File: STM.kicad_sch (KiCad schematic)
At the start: 29 parts, among them J7 PIN HEADER 2.54MM PITCH STR D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, U1 STM32L433CCU6, X1 CRYSTAL 32.0000MHZ 10PF SMD

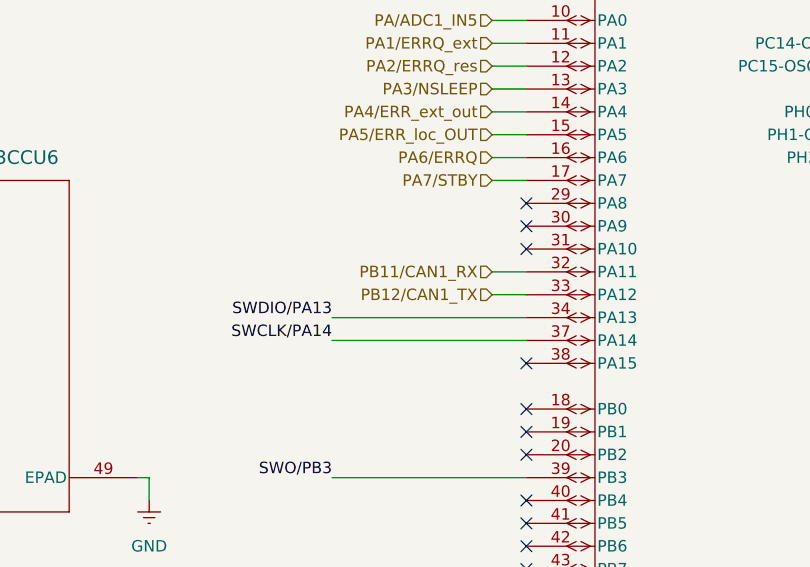
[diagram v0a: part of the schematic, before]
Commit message: minor changes
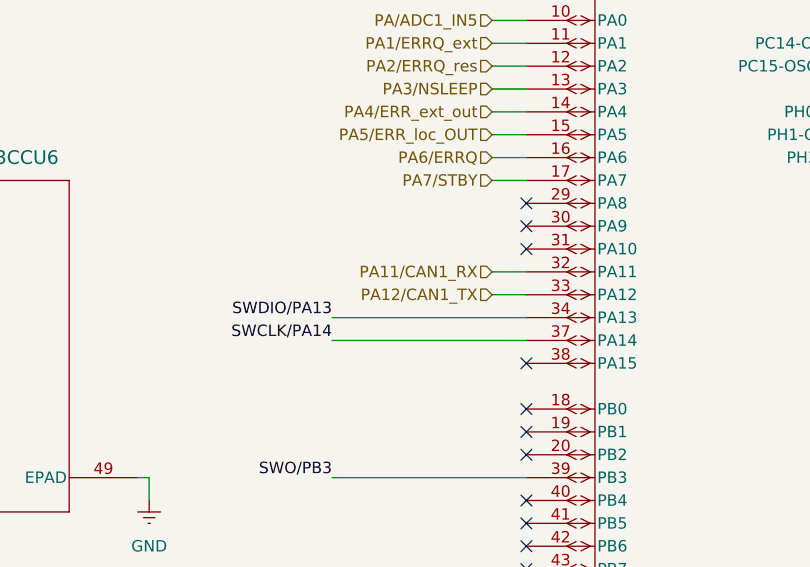
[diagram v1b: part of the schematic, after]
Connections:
- net PB11/CAN1_RX renamed PA11/CAN1_RX
- net PB12/CAN1_TX renamed PA12/CAN1_TX
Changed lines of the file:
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@@
 		)
 	)
-	(hierarchical_label "PB11{slash}CAN1_RX"
+	(hierarchical_label "PA11{slash}CAN1_RX"
 		(shape input)
 		(at 238.76 73.66 180)
@@
 		)
 	)
-	(hierarchical_label "PB12{slash}CAN1_TX"
+	(hierarchical_label "PA12{slash}CAN1_TX"
 		(shape input)
 		(at 238.76 76.2 180)

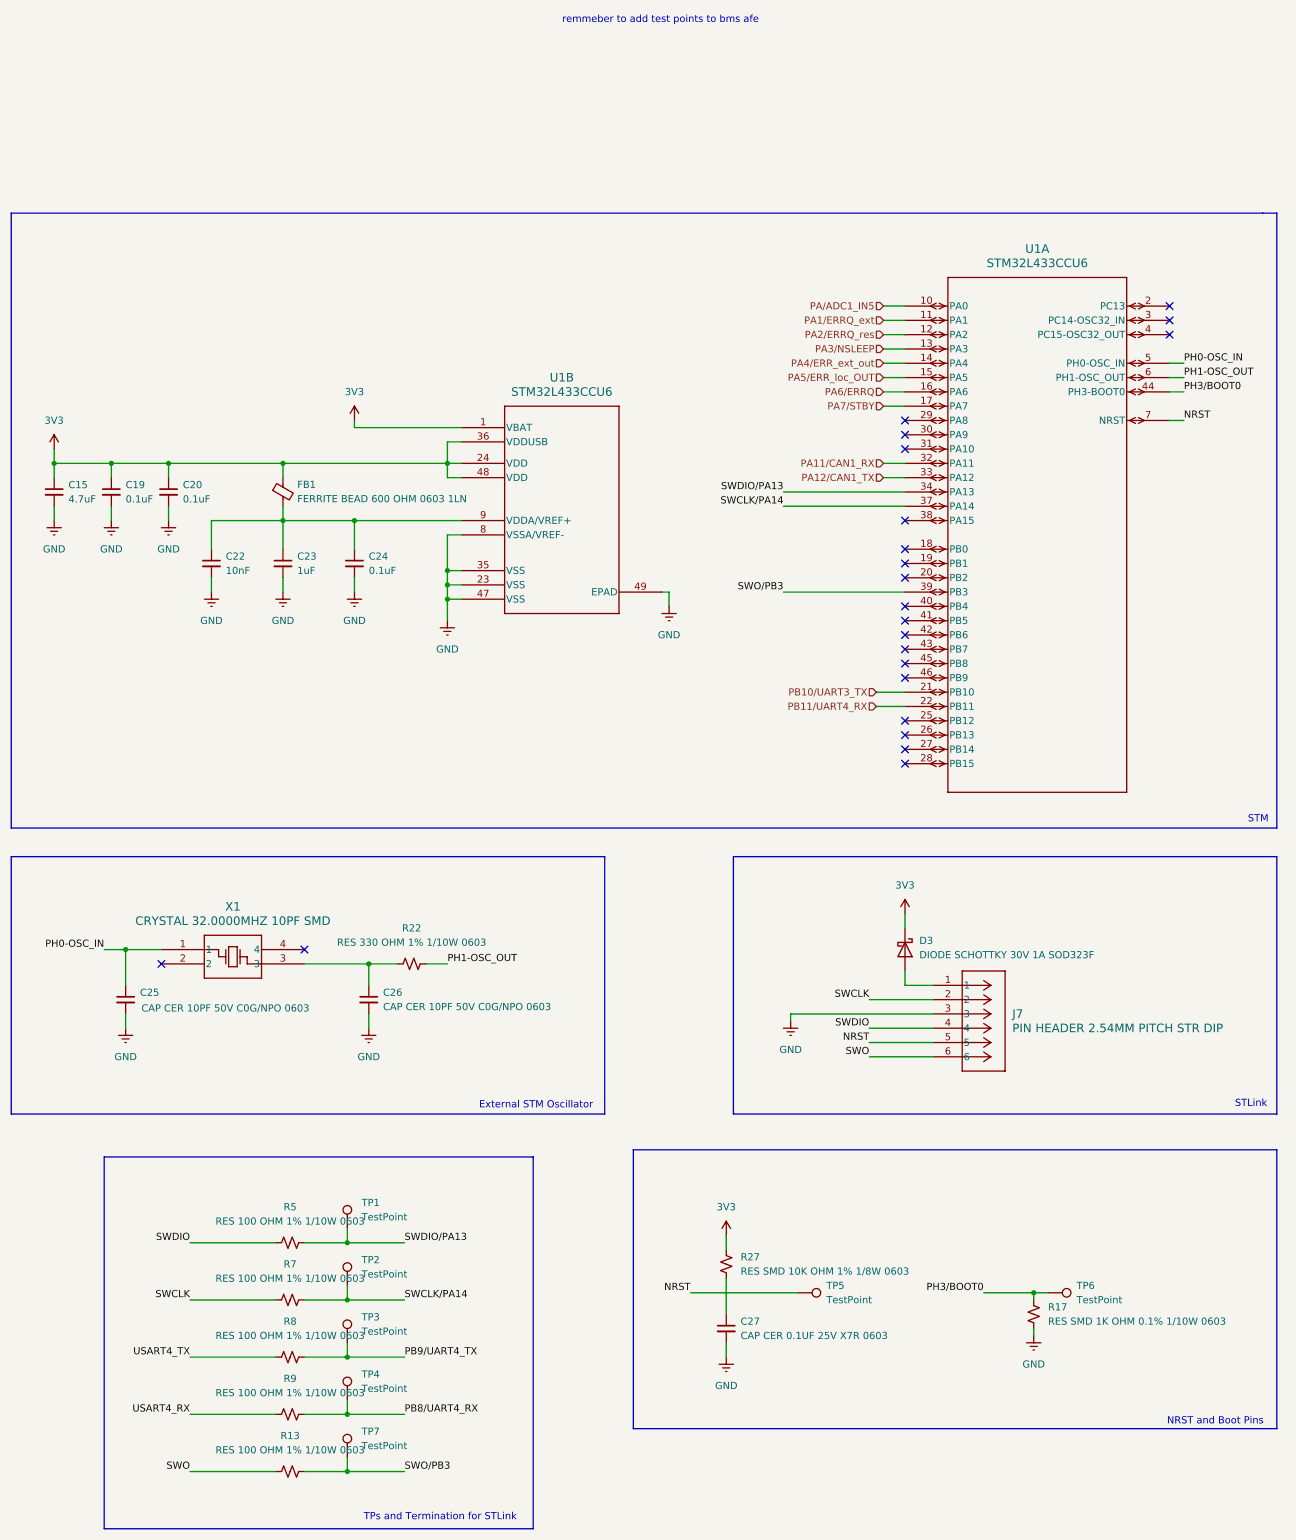
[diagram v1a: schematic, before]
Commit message: minor changes
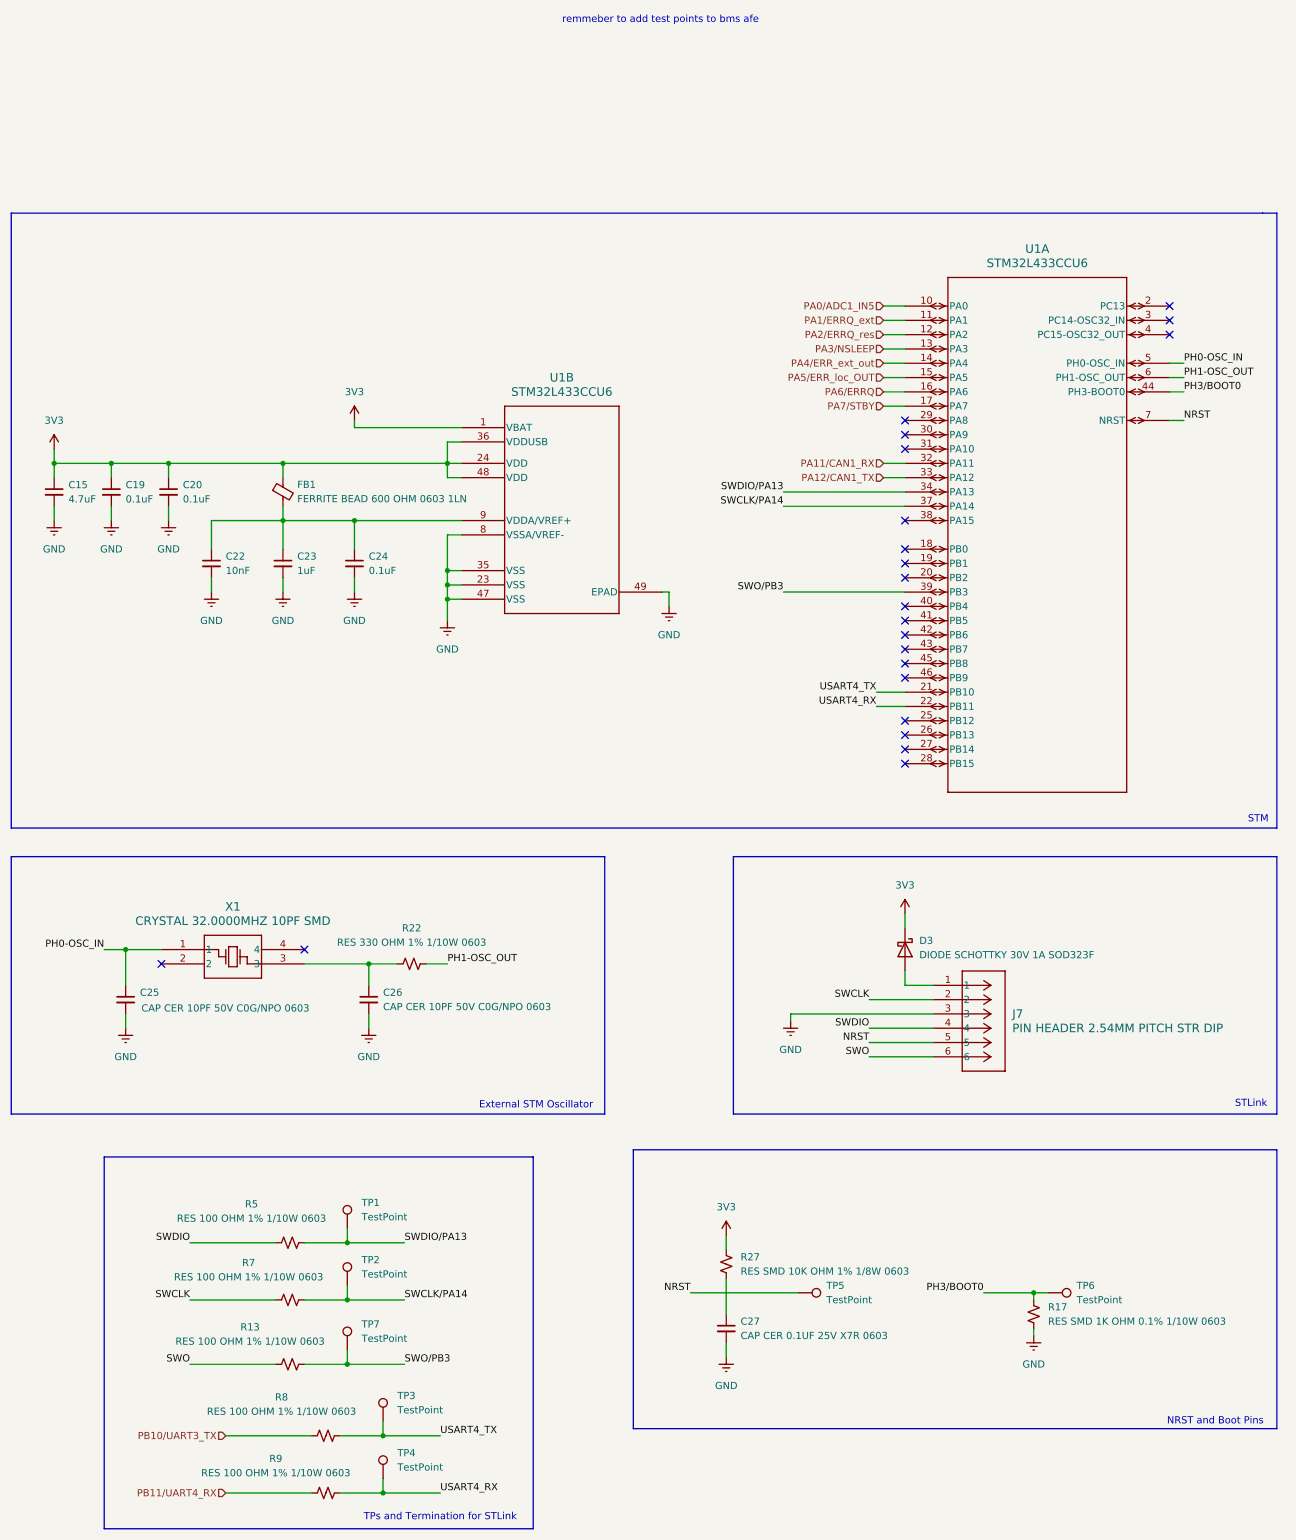
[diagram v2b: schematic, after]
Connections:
- net PB8/UART4_RX is gone; now on net USART4_RX: R9.2, TP4.1
- net PB9/UART4_TX is gone; now on net USART4_TX: R8.2, TP3.1
- net PB10/UART3_TX: now also R8.1; no longer U1.21 (PB10)
- net PB11/UART4_RX: now also R9.1; no longer U1.22 (PB11)
- net USART4_RX: now also U1.22 (PB11); no longer R9.1
- net USART4_TX: now also U1.21 (PB10); no longer R8.1
- net PA/ADC1_IN5 renamed PA0/ADC1_IN5
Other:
- moved on the sheet: R13, TP7
